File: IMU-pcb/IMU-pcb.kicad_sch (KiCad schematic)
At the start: 12 parts, among them J1 Conn_01x05_Female, U1 4056Board, U2 WeMos_D1_mini, U3 4754

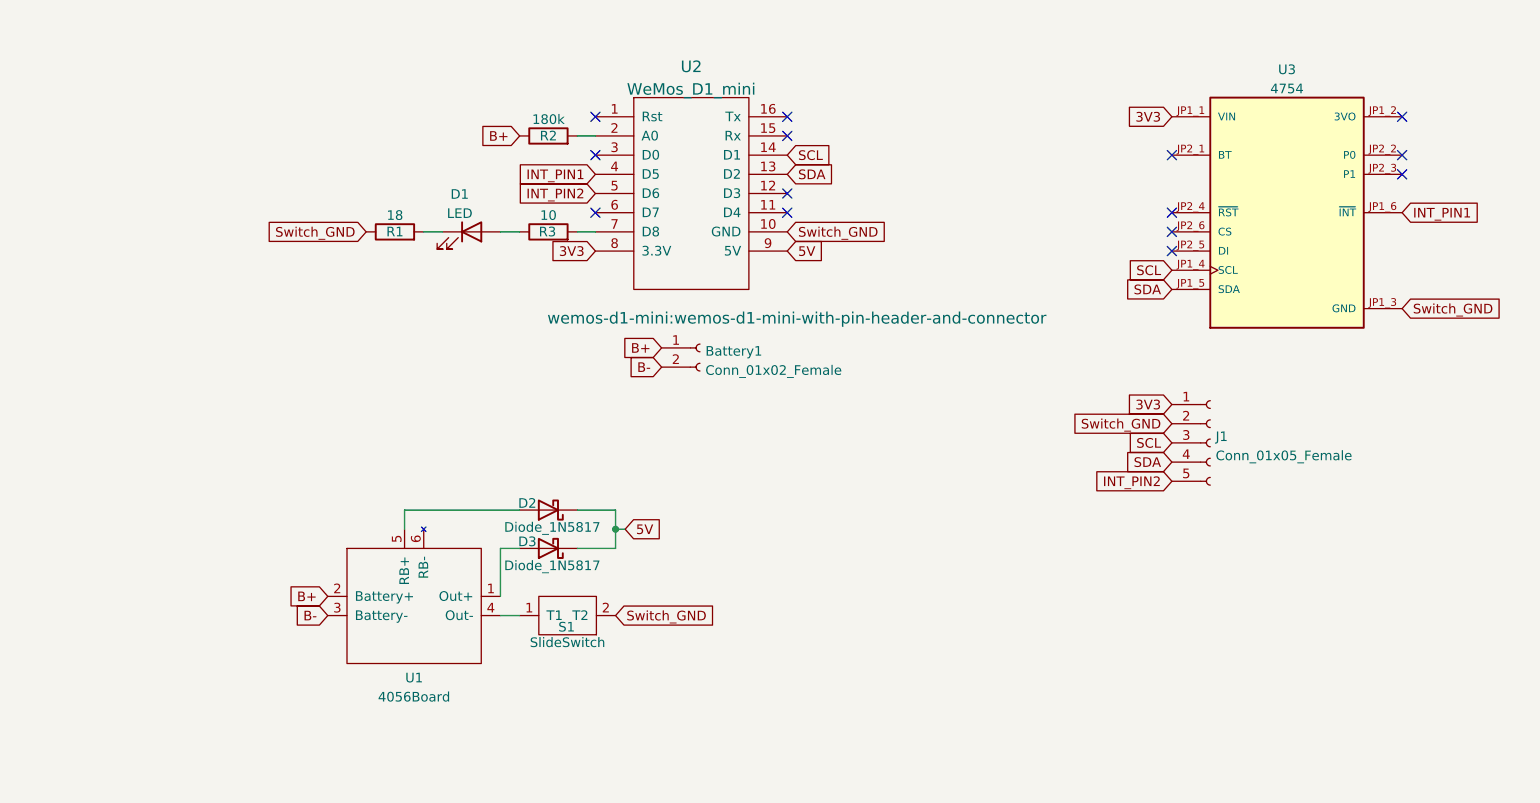
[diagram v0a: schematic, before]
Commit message: formalized schematic, symbols, and footprints
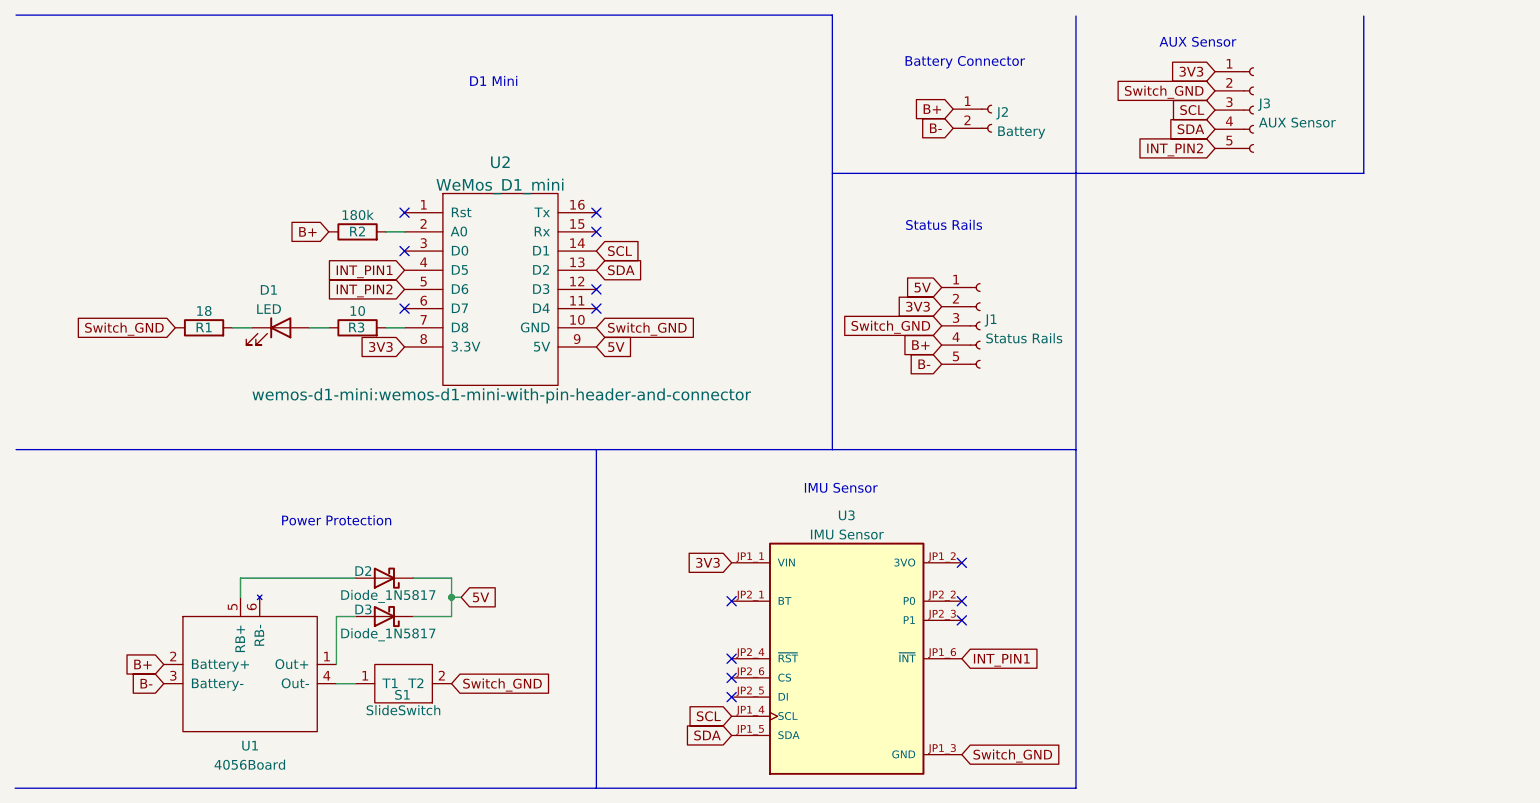
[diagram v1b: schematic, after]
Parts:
- added J1: Status Rails, bryx-comp-lib:fivePinConn, symbol Connector:Conn_01x05_Female
- J2: renamed from Battery1; value Conn_01x02_Female -> Battery
- J3: renamed from J1; value Conn_01x05_Female -> AUX Sensor
- U3: value 4754 -> IMU Sensor
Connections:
- net 3V3: now also J1.2 (Pin_2)
- net 5V: now also J1.1 (Pin_1)
- net B+: now also J1.4 (Pin_4)
- net B-: now also J1.5 (Pin_5)
- net Switch_GND: now also J1.3 (Pin_3)
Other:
- note added: "AUX Sensor"
- note added: "Battery Connector"
- note added: "D1 Mini"
- note added: "IMU Sensor"
- note added: "Power Protection"
- note added: "Status Rails"
- moved on the sheet: D1, D2, D3, J2, J3, R1, R2, R3, S1, U1, U2, U3
